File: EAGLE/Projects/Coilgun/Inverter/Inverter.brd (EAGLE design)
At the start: 43.2 x 79.4 mm, 18 parts, among them IC1 LM555CN, J1 XT30PW-M, J2 XT30PW-F, Q1 IRF840, Q2 IRF9530, Q3 IRF840, Q4 IRF9530, U1 MIC4422, U2 MIC4421

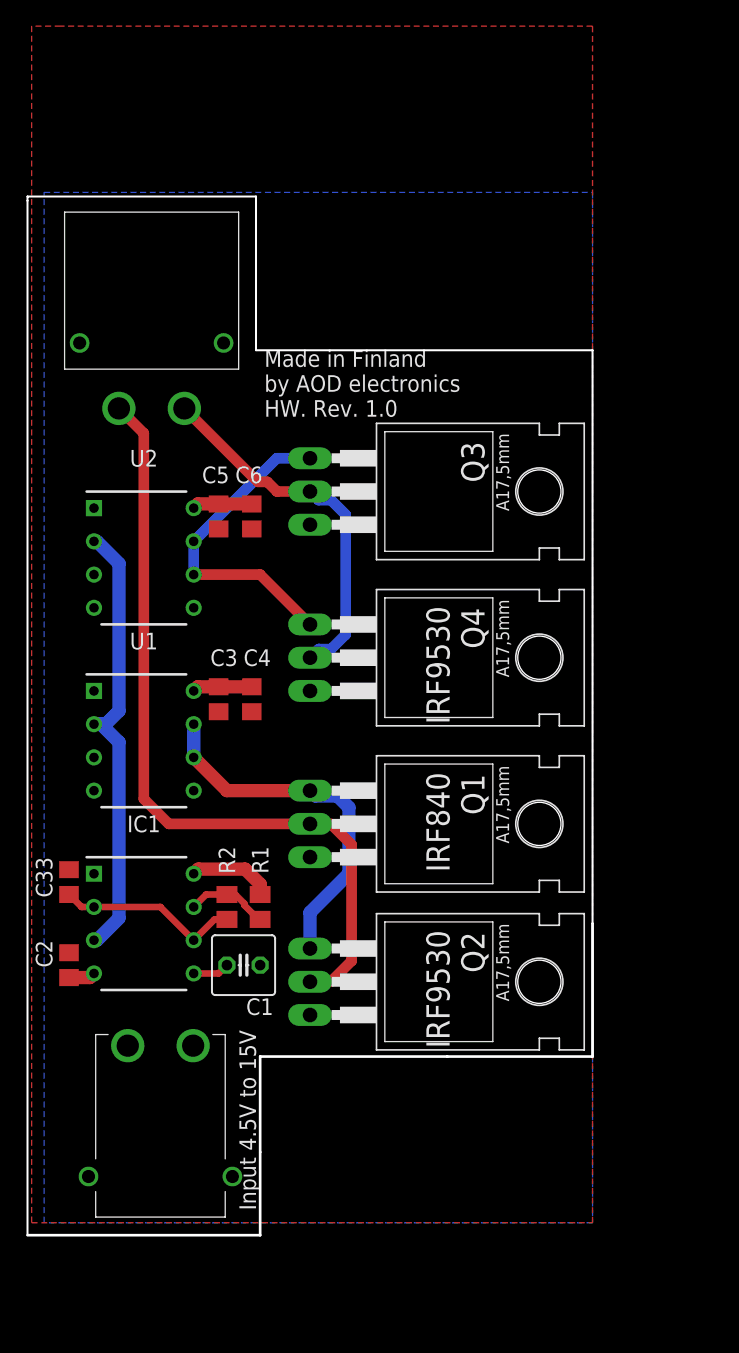
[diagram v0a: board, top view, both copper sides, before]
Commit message: Add latest mods
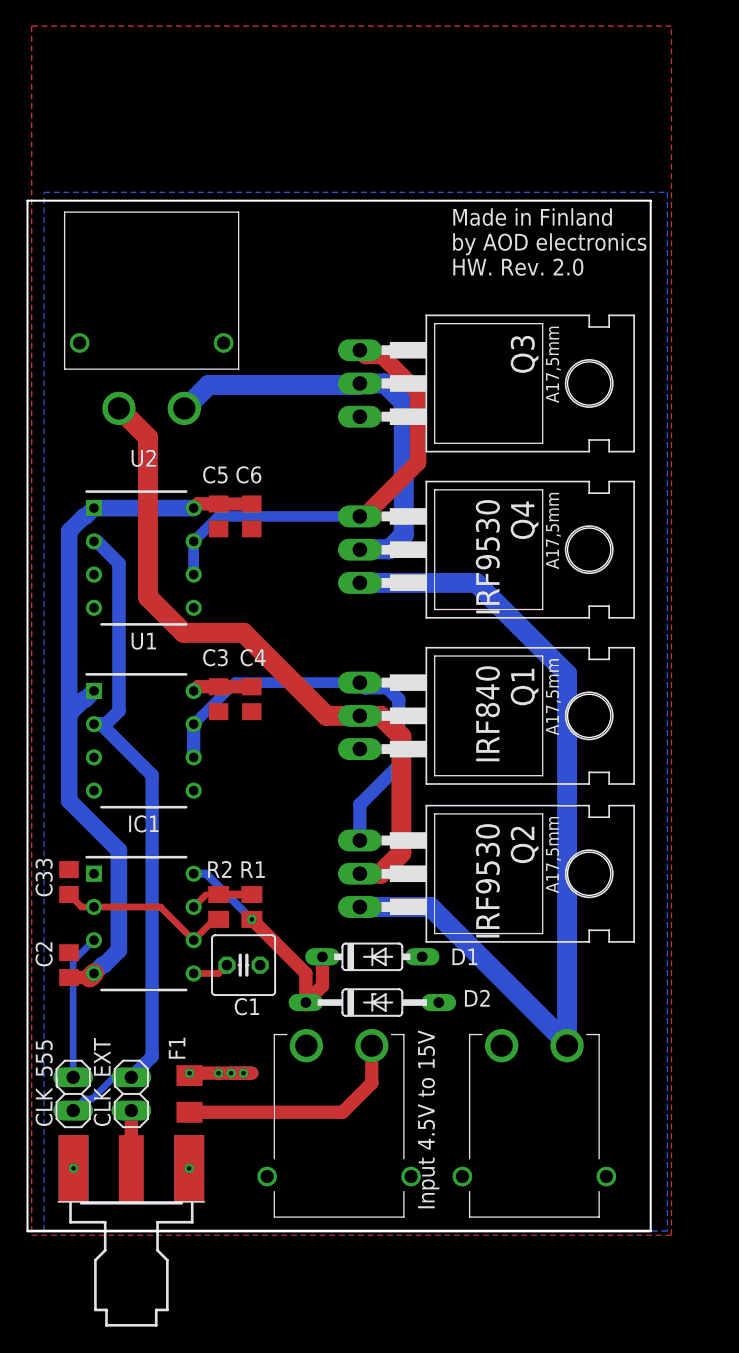
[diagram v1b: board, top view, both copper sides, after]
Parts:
- added CLK_555, CLK_EXT: (no value), pinhead:1X02
- added D1: 1N4148DO35-7, diode:DO35-7
- added D2: (no value), diode:DO35Z10
- added F1: 0.2 A, rcl:M1206
- added J3: XT30PW-M, XT30PW-M:XT30PWM
- added X1: SMA-142-0711-871/876, con-coax:J502-ND-142-0711-871/876
- moved J1 13.7 mm to (23.2, 7.62)
- moved Q2 9.09 mm to (31.1, 26.7)
- moved Q3 9.09 mm to (31.1, 64.1)
- moved Q4 9.09 mm to (31.1, 51.4)
- moved Q1 9.09 mm to (31.1, 38.7)
- moved R2 0.63 mm to (14.0, 24.1)
- moved R1 0.63 mm to (16.5, 24.1), turned to 270 degrees
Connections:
- net N$10 renamed DRIVE_INV
- net N$9 renamed DRIVE_NON
- removed net N$8: IC1.3, U1.2, U2.2
- new net CLK: CLK_555.2, CLK_EXT.2, U1.2, U2.2
- new net CLK_555: CLK_555.1, IC1.3
- new net CLK_EXT: CLK_EXT.1, X1.1
- new net N$11: F1.1, J1.1
- new net VS: J3.1, Q2.3, Q4.3
- net GND: now also D1.A, D2.A, J3.2, X1.G@1, X1.G@2, X1.G@3, X1.G@4
- net VCC: now also D1.C, D2.C, F1.2; no longer J1.1, Q2.3, Q4.3
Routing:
- net VS: track 0.00 -> 67.3 mm
- net VCC: track 17.7 -> 84.9 mm, vias 0 -> 5
- net CLK: track 0.00 -> 51.5 mm
- net N$8: track 34.8 -> 0.00 mm
- net N$11: track 0.00 -> 17.7 mm
- net CLK_555: track 0.00 -> 11.1 mm
- net N$4: track 60.7 -> 51.8 mm
- net DRIVE_INV: track 24.5 -> 33.3 mm
- net CLK_EXT: track 0.00 -> 6.01 mm
- net DRIVE_NON: track 28.0 -> 32.1 mm
- net N$5: track 28.3 -> 32.1 mm
- net N$2: track 6.34 -> 4.84 mm
- net N$1: track 14.2 -> 13.5 mm
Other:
- board size 43.2 x 79.4 mm -> 47.6 x 78.7 mm
- board text added: "Made in Finland by AOD electronics HW. Rev. 2.0"
- board text removed: "Made in Finland by AOD electronics HW. Rev. 1.0"
